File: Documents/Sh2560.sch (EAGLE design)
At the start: 5 parts, among them CN1 22-23-2051

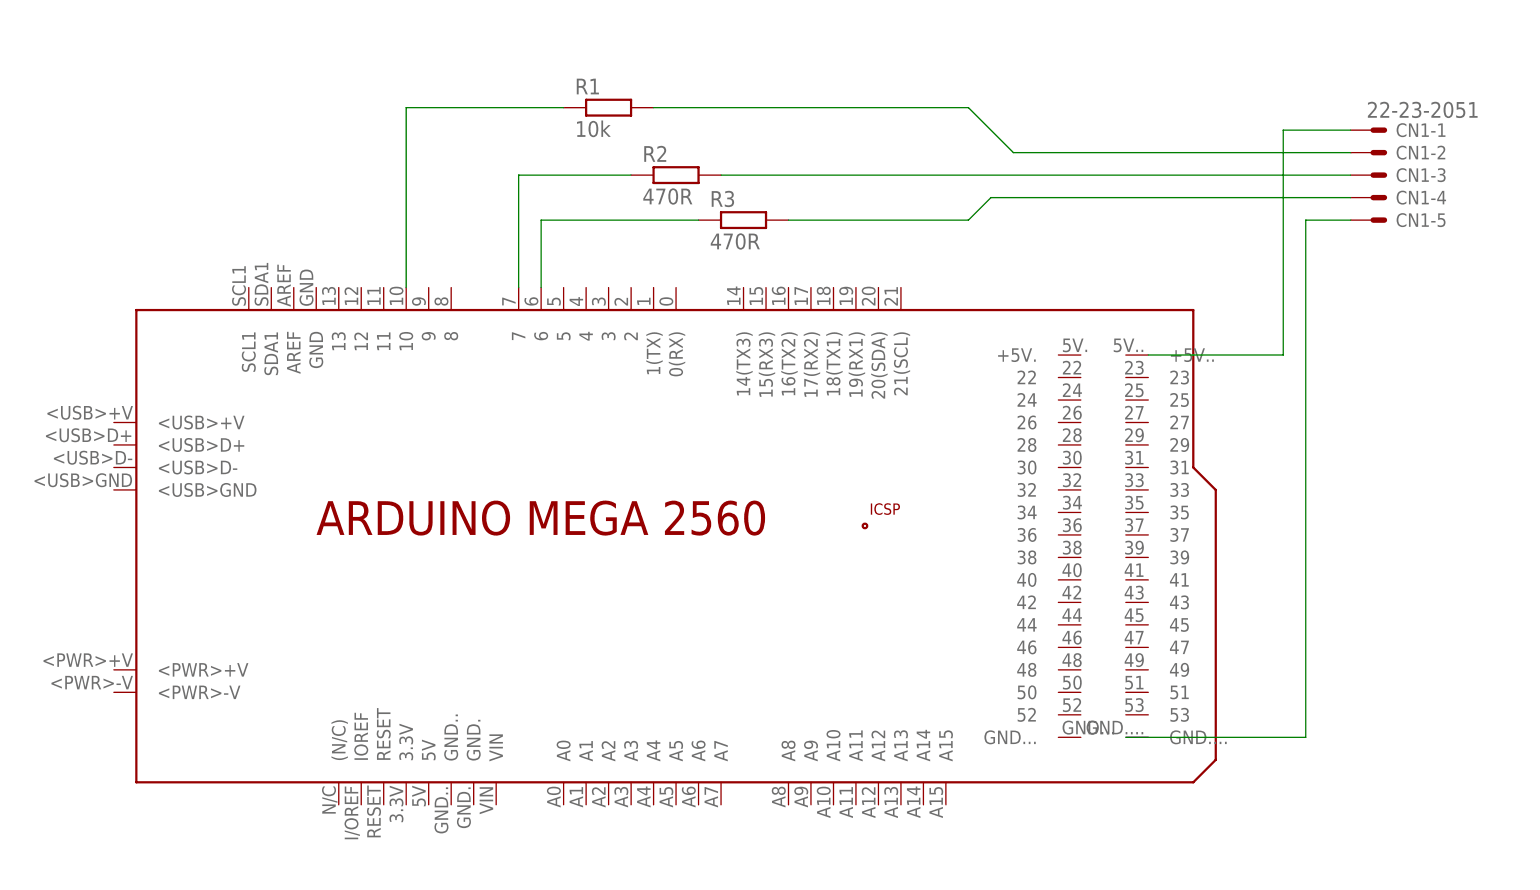
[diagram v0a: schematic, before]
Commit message: Add pdf
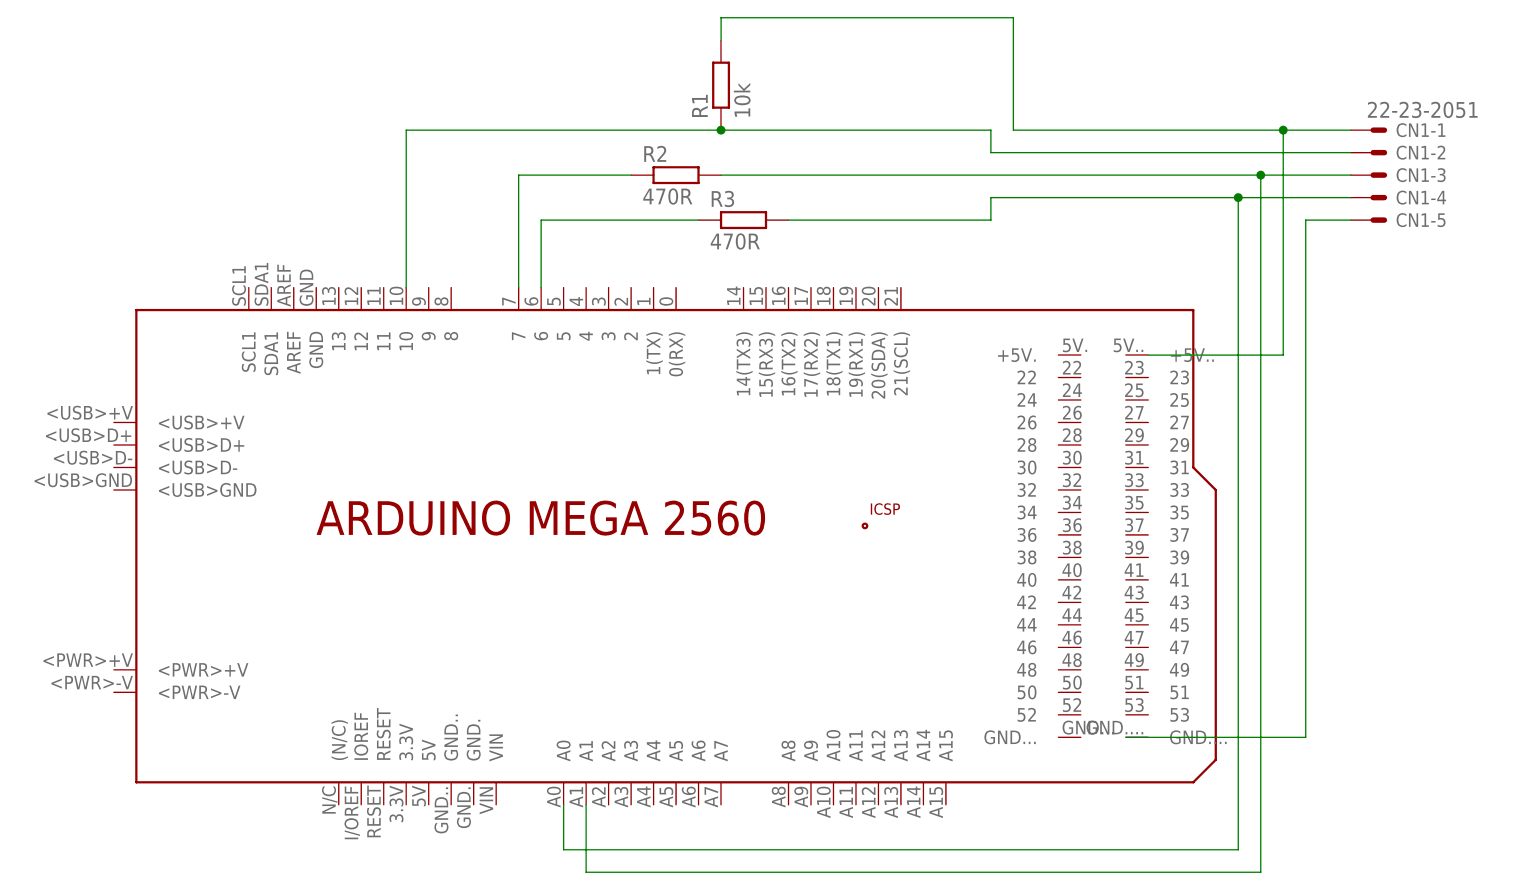
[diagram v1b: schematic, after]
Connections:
- removed net N$8: CN1-2.S, R1.2
- net N$3: now also CN1-2.S
- net N$5: now also R1.2
- net N$6: now also PCB1.A0
- net N$7: now also PCB1.A1
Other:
- moved on the sheet: R1
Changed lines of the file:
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@@
 <instances>
 <instance part="PCB1" gate="G$1" x="83.82" y="33.02"/>
-<instance part="R1" gate="G$1" x="78.74" y="81.28"/>
+<instance part="R1" gate="G$1" x="91.44" y="83.82" rot="R90"/>
 <instance part="R2" gate="G$1" x="86.36" y="73.66"/>
 <instance part="R3" gate="G$1" x="93.98" y="68.58"/>
@@
 <pinref part="R1" gate="G$1" pin="1"/>
 <pinref part="PCB1" gate="G$1" pin="10"/>
-<wire x1="73.66" y1="81.28" x2="55.88" y2="81.28" width="0.1524" layer="91"/>
-<wire x1="55.88" y1="81.28" x2="55.88" y2="60.96" width="0.1524" layer="91"/>
+<wire x1="91.44" y1="78.74" x2="55.88" y2="78.74" width="0.1524" layer="91"/>
+<wire x1="55.88" y1="78.74" x2="55.88" y2="60.96" width="0.1524" layer="91"/>
+<wire x1="91.44" y1="78.74" x2="121.92" y2="78.74" width="0.1524" layer="91"/>
+<wire x1="121.92" y1="78.74" x2="121.92" y2="76.2" width="0.1524" layer="91"/>
+<junction x="91.44" y="78.74"/>
+<pinref part="CN1" gate="-2" pin="S"/>
+<wire x1="121.92" y1="76.2" x2="162.56" y2="76.2" width="0.1524" layer="91"/>
 </segment>
 </net>
@@
 <pinref part="CN1" gate="-1" pin="S"/>
 <wire x1="154.94" y1="78.74" x2="162.56" y2="78.74" width="0.1524" layer="91"/>
-</segment>
-</net>
-<net name="N$6" class="0">
-<segment>
-<pinref part="CN1" gate="-4" pin="S"/>
-<wire x1="162.56" y1="71.12" x2="121.92" y2="71.12" width="0.1524" layer="91"/>
-<pinref part="R3" gate="G$1" pin="2"/>
-<wire x1="121.92" y1="71.12" x2="119.38" y2="68.58" width="0.1524" layer="91"/>
-<wire x1="119.38" y1="68.58" x2="99.06" y2="68.58" width="0.1524" layer="91"/>
+<pinref part="R1" gate="G$1" pin="2"/>
+<wire x1="91.44" y1="88.9" x2="91.44" y2="91.44" width="0.1524" layer="91"/>
+<wire x1="91.44" y1="91.44" x2="124.46" y2="91.44" width="0.1524" layer="91"/>
+<wire x1="124.46" y1="91.44" x2="124.46" y2="78.74" width="0.1524" layer="91"/>
+<wire x1="124.46" y1="78.74" x2="154.94" y2="78.74" width="0.1524" layer="91"/>
+<junction x="154.94" y="78.74"/>
 </segment>
 </net>
@@
 <pinref part="R2" gate="G$1" pin="2"/>
 <pinref part="CN1" gate="-3" pin="S"/>
-<wire x1="91.44" y1="73.66" x2="162.56" y2="73.66" width="0.1524" layer="91"/>
+<wire x1="91.44" y1="73.66" x2="152.4" y2="73.66" width="0.1524" layer="91"/>
+<wire x1="152.4" y1="73.66" x2="162.56" y2="73.66" width="0.1524" layer="91"/>
+<wire x1="152.4" y1="73.66" x2="152.4" y2="-5.08" width="0.1524" layer="91"/>
+<junction x="152.4" y="73.66"/>
+<wire x1="152.4" y1="-5.08" x2="76.2" y2="-5.08" width="0.1524" layer="91"/>
+<pinref part="PCB1" gate="G$1" pin="A1"/>
+<wire x1="76.2" y1="-5.08" x2="76.2" y2="2.54" width="0.1524" layer="91"/>
 </segment>
 </net>
-<net name="N$8" class="0">
+<net name="N$6" class="0">
 <segment>
-<pinref part="R1" gate="G$1" pin="2"/>
-<wire x1="83.82" y1="81.28" x2="119.38" y2="81.28" width="0.1524" layer="91"/>
-<wire x1="119.38" y1="81.28" x2="124.46" y2="76.2" width="0.1524" layer="91"/>
-<pinref part="CN1" gate="-2" pin="S"/>
-<wire x1="124.46" y1="76.2" x2="162.56" y2="76.2" width="0.1524" layer="91"/>
+<pinref part="R3" gate="G$1" pin="2"/>
+<wire x1="99.06" y1="68.58" x2="121.92" y2="68.58" width="0.1524" layer="91"/>
+<wire x1="121.92" y1="68.58" x2="121.92" y2="71.12" width="0.1524" layer="91"/>
+<pinref part="CN1" gate="-4" pin="S"/>
+<wire x1="121.92" y1="71.12" x2="149.86" y2="71.12" width="0.1524" layer="91"/>
+<wire x1="149.86" y1="71.12" x2="162.56" y2="71.12" width="0.1524" layer="91"/>
+<wire x1="149.86" y1="71.12" x2="149.86" y2="-2.54" width="0.1524" layer="91"/>
+<junction x="149.86" y="71.12"/>
+<wire x1="149.86" y1="-2.54" x2="73.66" y2="-2.54" width="0.1524" layer="91"/>
+<pinref part="PCB1" gate="G$1" pin="A0"/>
+<wire x1="73.66" y1="-2.54" x2="73.66" y2="2.54" width="0.1524" layer="91"/>
 </segment>
 </net>
